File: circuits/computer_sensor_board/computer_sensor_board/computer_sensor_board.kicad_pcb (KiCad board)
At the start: 2 copper layers, 70 x 35 mm, 17 parts, among them J1 Conn_Switching_Hub, J2 Conn_Jetson, J5 Conn_VLP16, J6 Conn_Main_DCDC, J7 Conn_Router, Q2 2SJ555-E

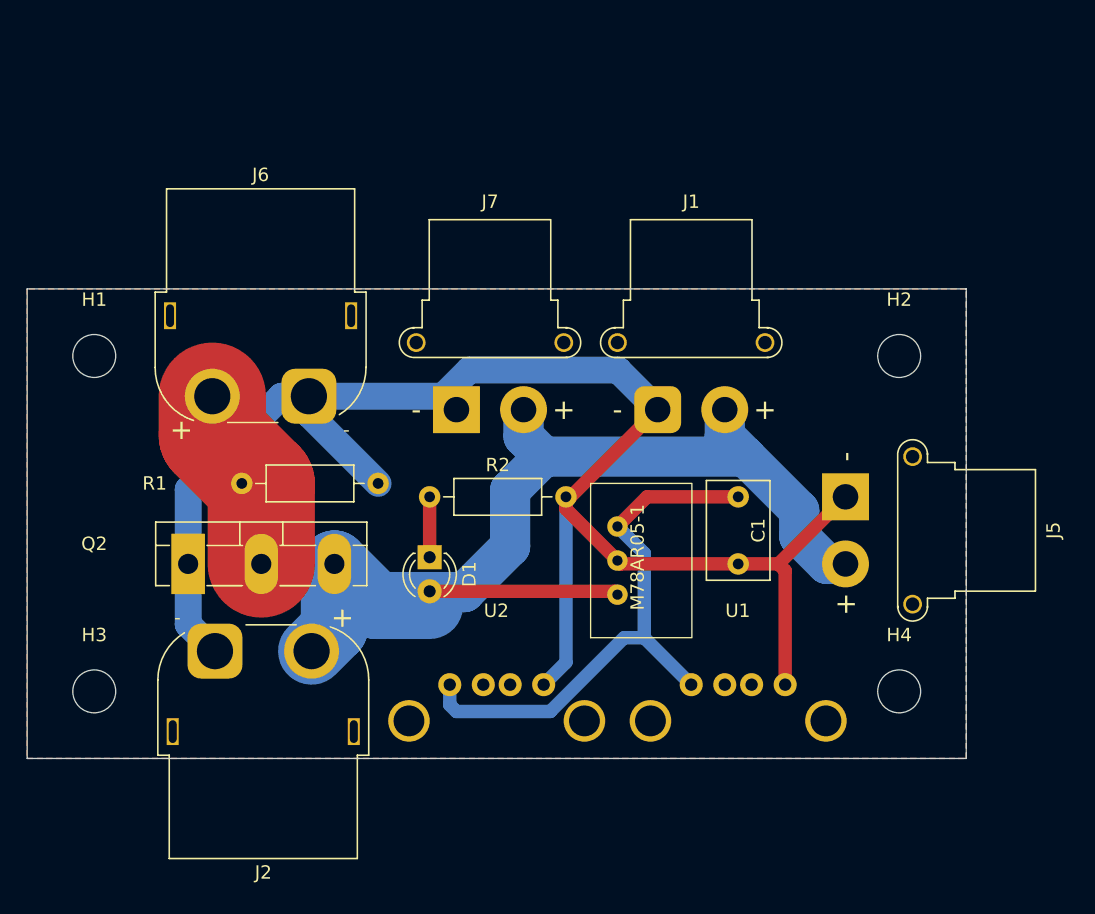
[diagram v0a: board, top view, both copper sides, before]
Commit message: add heatsink
Signed-off-by: Masaya Kataoka <ms.kataoka@gmail.com>
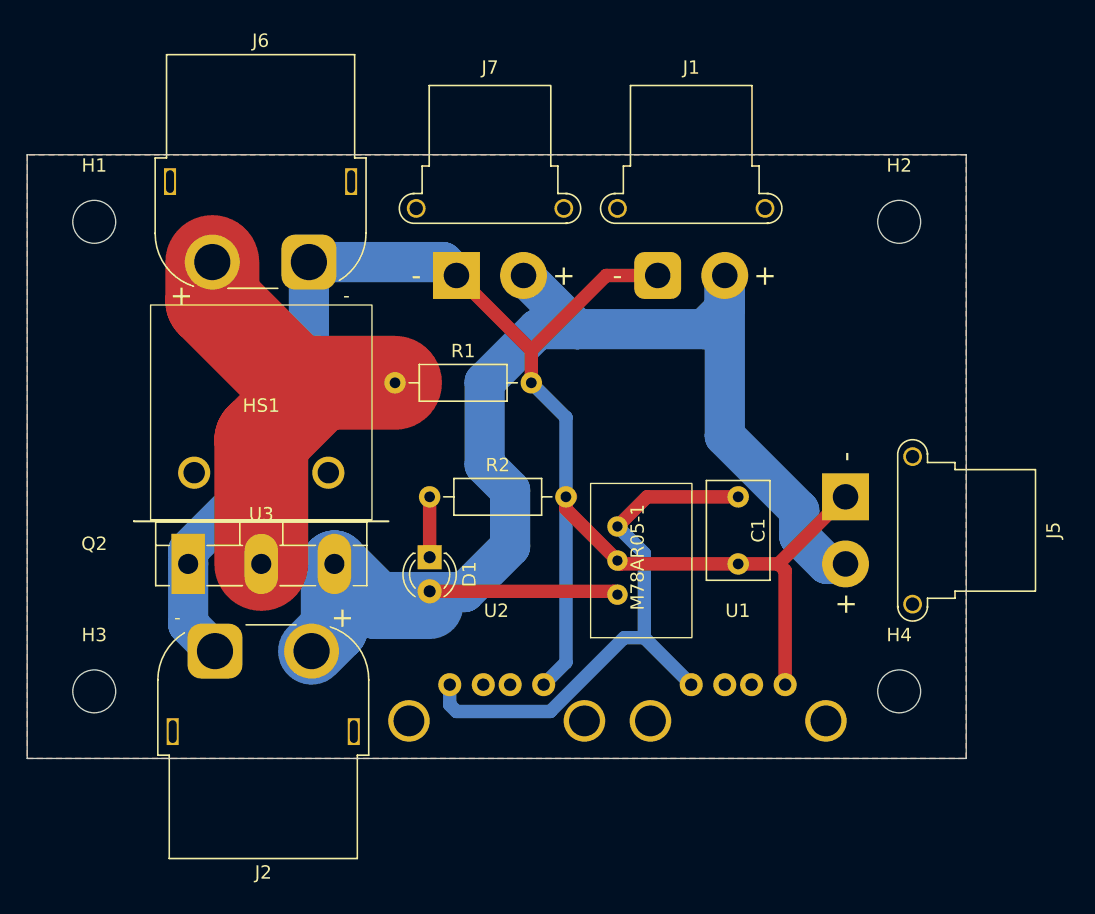
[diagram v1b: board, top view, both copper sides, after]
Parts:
- added HS1: Heatsink, 16PB017-01025:16PB017-01025, F.Cu at (187.4, 64.2)
- added U3: Heatsink_sheet, 16PB017-01025:TO-3PH, F.Cu at (187.4, 72.3)
- J2: value Conn_Jetson -> Jetson
- J6: value Conn_Main_DCDC -> Main_DCDC
- moved R1 13.7 mm to (197.4, 62.0)
- moved H1 10.0 mm to (175.0, 50.0)
- moved H2 10.0 mm to (235.0, 50.0)
- moved J1 10.0 mm to (217.0, 54.0)
- moved J6 10.0 mm to (191.0, 53.0)
- moved J7 10.0 mm to (202.0, 54.0)
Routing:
- net Net-(D1-A): track 80.0 -> 104.5 mm
- net Net-(J6-Pin_2): track 14.0 -> 34.3 mm
- net GND: track 123.5 -> 126.7 mm
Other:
- board size 70 x 35 mm -> 70 x 45 mm
